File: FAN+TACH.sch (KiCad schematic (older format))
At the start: 6 parts, among them Q2 2N7002, Q3 2N7002, Q4 2N7002

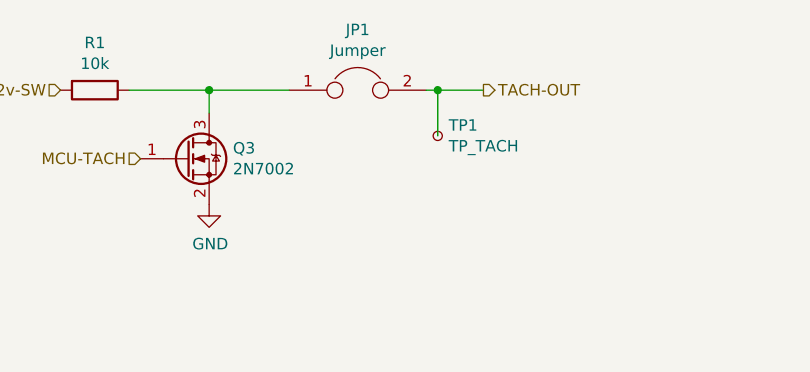
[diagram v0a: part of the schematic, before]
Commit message: Finish reroute again
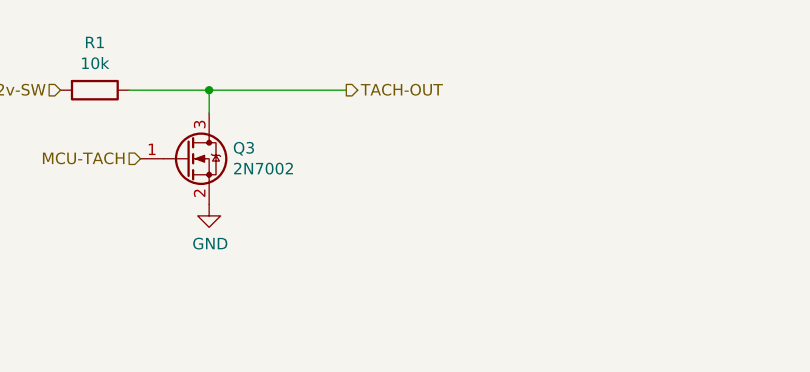
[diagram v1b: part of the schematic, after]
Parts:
- removed JP1: Jumper, Jumper:SolderJumper-2_P1.3mm_Open_RoundedPad1.0x1.5mm, symbol Device:Jumper
- removed TP1: TP_TACH, TestPoint:TestPoint_Pad_D1.0mm, symbol Connector:TestPoint_Small
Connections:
- net TACH-OUT: now also Q3.3 (D), R1.1
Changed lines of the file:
@@
 Comment4 ""
 $EndDescr
-Text HLabel 3900 2850 2    50   Output ~ 0
+Text HLabel 3300 2850 2    50   Output ~ 0
 TACH-OUT
-$Comp
-L Device:Jumper JP1
-U 1 1 5EFA7131
-P 3350 2850
-F 0 "JP1" H 3350 3114 50  0000 C CNN
-F 1 "Jumper" H 3350 3023 50  0000 C CNN
-F 2 "Jumper:SolderJumper-2_P1.3mm_Open_RoundedPad1.0x1.5mm" H 3350 2850 50  0001 C CNN
-F 3 "~" H 3350 2850 50  0001 C CNN
-	1    3350 2850
-	1    0    0    -1
-$EndComp
-$Comp
-L Connector:TestPoint_Small TP1
-U 1 1 60D91417
-P 3700 3050
-F 0 "TP1" H 3748 3096 50  0000 L CNN
-F 1 "TP_TACH" H 3748 3005 50  0000 L CNN
-F 2 "TestPoint:TestPoint_Pad_D1.0mm" H 3900 3050 50  0001 C CNN
-F 3 "~" H 3900 3050 50  0001 C CNN
-	1    3700 3050
-	1    0    0    -1
-$EndComp
-Wire Wire Line
-	3700 3050 3700 2850
-Wire Wire Line
-	3650 2850 3700 2850
-Connection ~ 3700 2850
-Wire Wire Line
-	3700 2850 3900 2850
 $Comp
 L Transistor_FET:2N7002 Q2
@@
 	1    0    0    -1
 $EndComp
-Wire Wire Line
-	2700 2850 3050 2850
 Connection ~ 2700 2850
 Text HLabel 2400 3150 0    50   Input ~ 0
@@
 	1    0    0    -1
 $EndComp
+Wire Wire Line
+	2700 2850 3300 2850
 $EndSCHEMATC
